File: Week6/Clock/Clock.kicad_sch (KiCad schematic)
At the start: 53 parts, among them J1 Power_inlet_vertical, J2 Conn_01x06, SW1 RotaryEncoder_Switch, SW2 Omron_B3F_SPST, U1 L7805, U2 ATmega328-PU, U4 DS1307_DIP-8, U5 MAX7219, U6 MAX7219, Y1 Crystal 16MHZ, Y2 Crystal_32768Hz

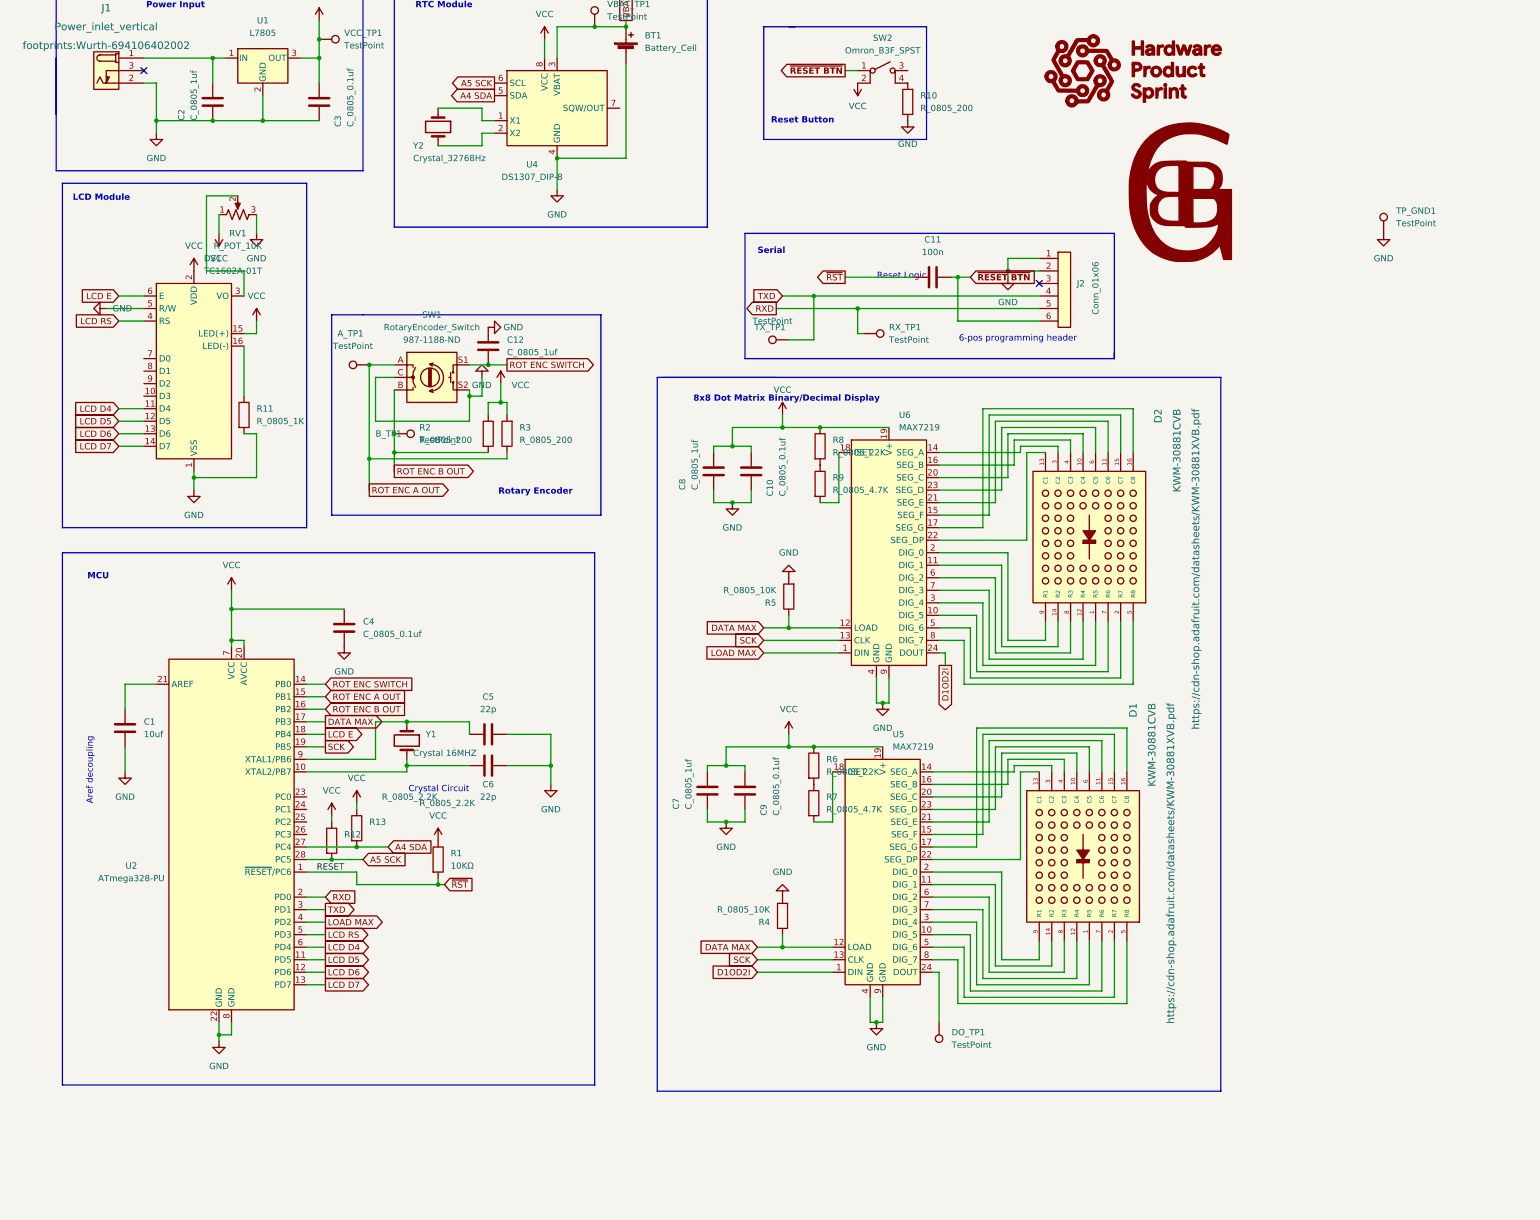
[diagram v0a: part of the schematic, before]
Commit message: Uploaded Student Designs :)
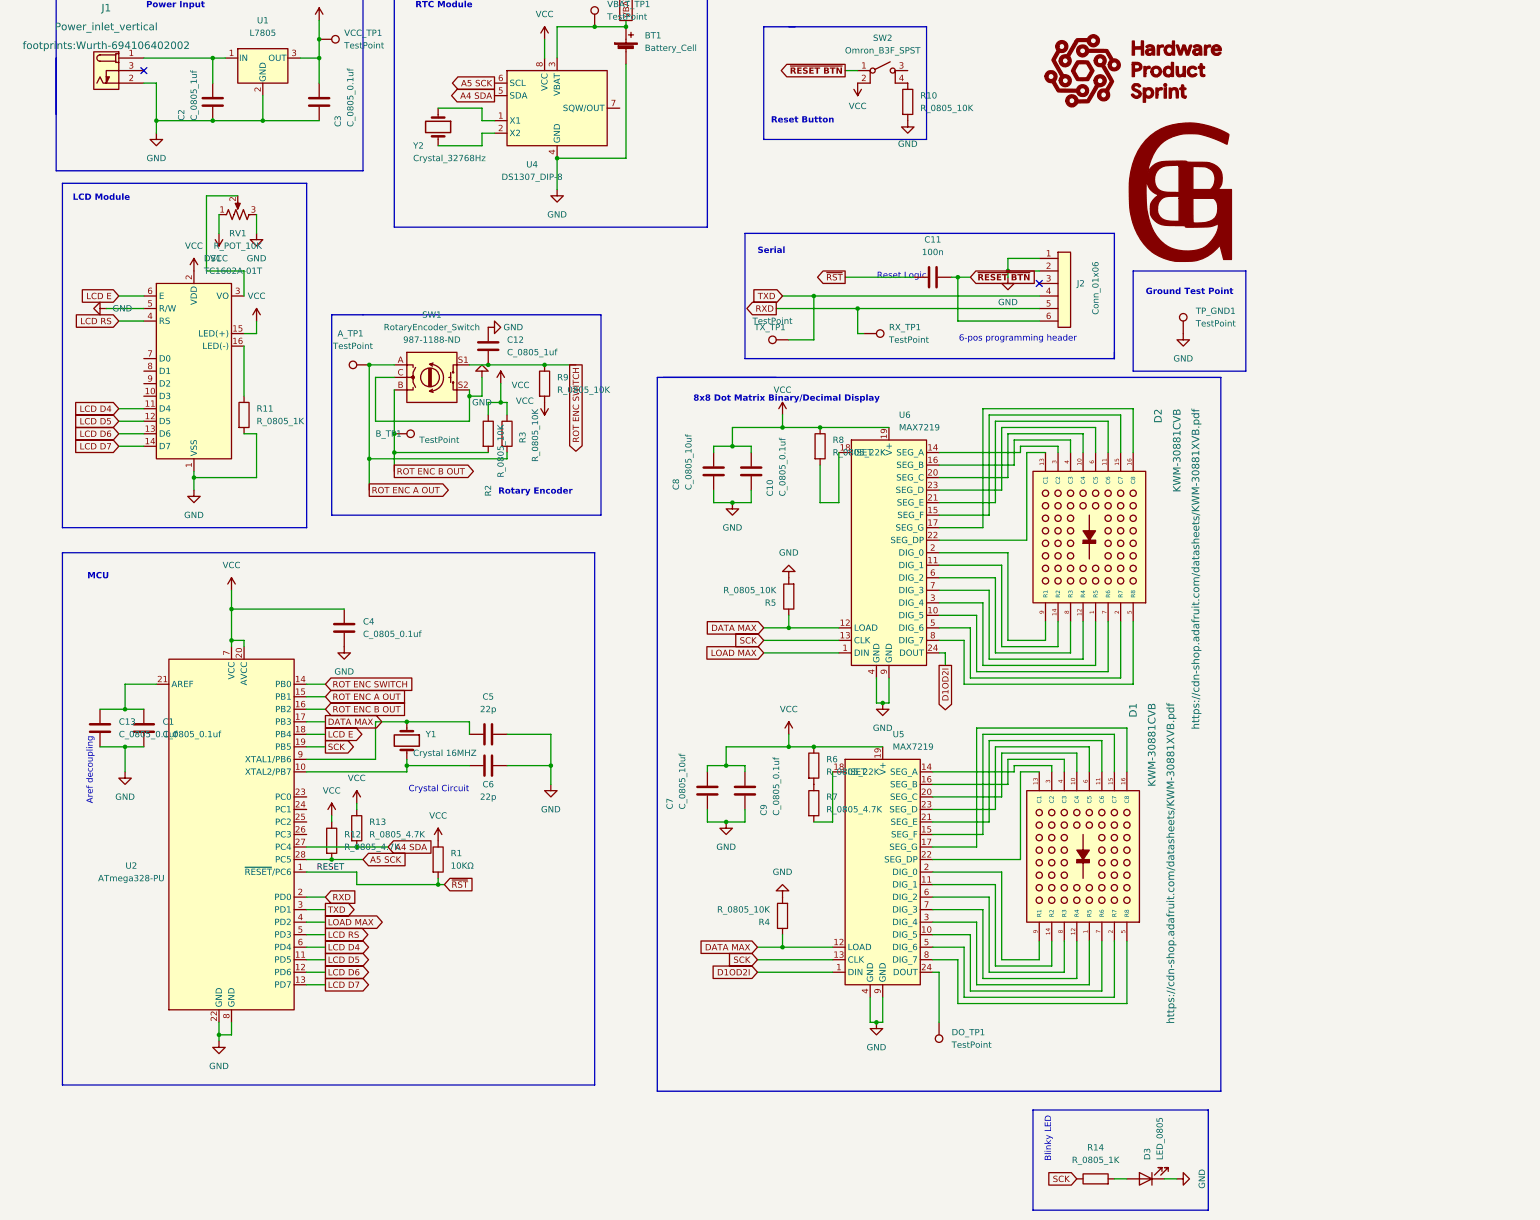
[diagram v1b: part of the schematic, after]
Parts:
- removed C1: 10uf, footprints:C_0805_2012Metric, symbol HPS:C_0805_10uf
- removed C7, C8: C_0805_1uf, footprints:C_0805_2012Metric, symbol HPS:C_0805_1uf
- removed R10, R2, R3: R_0805_200, footprints:R_0805_2012Metric, symbol HPS:R_0805_1K
- removed R12, R13: R_0805_2.2K, footprints:R_0805_2012Metric, symbol HPS:R_0805_2.2K
- removed R9: R_0805_4.7K, footprints:R_0805_2012Metric, symbol HPS:R_0805_4.7K
- added C1, C13: C_0805_0.1uf, footprints:C_0805_2012Metric, symbol HPS:C_0805_0.1uf
- added C7, C8: C_0805_10uf, footprints:C_0805_2012Metric, symbol HPS:C_0805_10uf
- added D3: LED_0805, footprints:LED_0805_2012Metric, symbol HPS:LED_0805
- added R10, R2, R3, R9: R_0805_10K, footprints:R_0805_2012Metric, symbol HPS:R_0805_10K
- added R12, R13: R_0805_4.7K, footprints:R_0805_2012Metric, symbol HPS:R_0805_4.7K
- added R14: R_0805_1K, footprints:R_0805_2012Metric, symbol HPS:R_0805_1K
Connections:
- net A4 SDA: now also R13.2
- net A5 SCK: now also R12.2
- net GND: now also C1.2, C13.2, C7.2, C8.2, D3.1 (K), R10.2
- net ROT ENC A OUT: now also R3.2
- net ROT ENC B OUT: now also R2.2
- net ROT ENC SWITCH: now also R9.1
- net SCK: now also R14.1
- net VCC: now also C7.1, C8.1, R12.1, R13.1, R2.1, R3.1, R9.2
- net at U2.21 (AREF): now also C1.1, C13.1
- net at SW2.4 (B): now also R10.1
- net at R8.2: now also U6.18 (ISET)
- new net: D3.2 (A), R14.2
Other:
- note added: "Blinky LED"
- note added: "Ground Test Point"
- moved on the sheet: TP_GND1
